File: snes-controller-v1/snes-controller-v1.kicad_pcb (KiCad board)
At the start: 2 copper layers, 66.1 x 20.1 mm, 19 parts, among them J1 USB_B_Micro, J2 NES, J3 Conn_01x06, J4 SNES_Controller_Socket, J5 SNES_Controller_Socket, U1 SN74LVC125ADR, U2 AP2112K-3.3, U7 ATSAMD21E18A-A

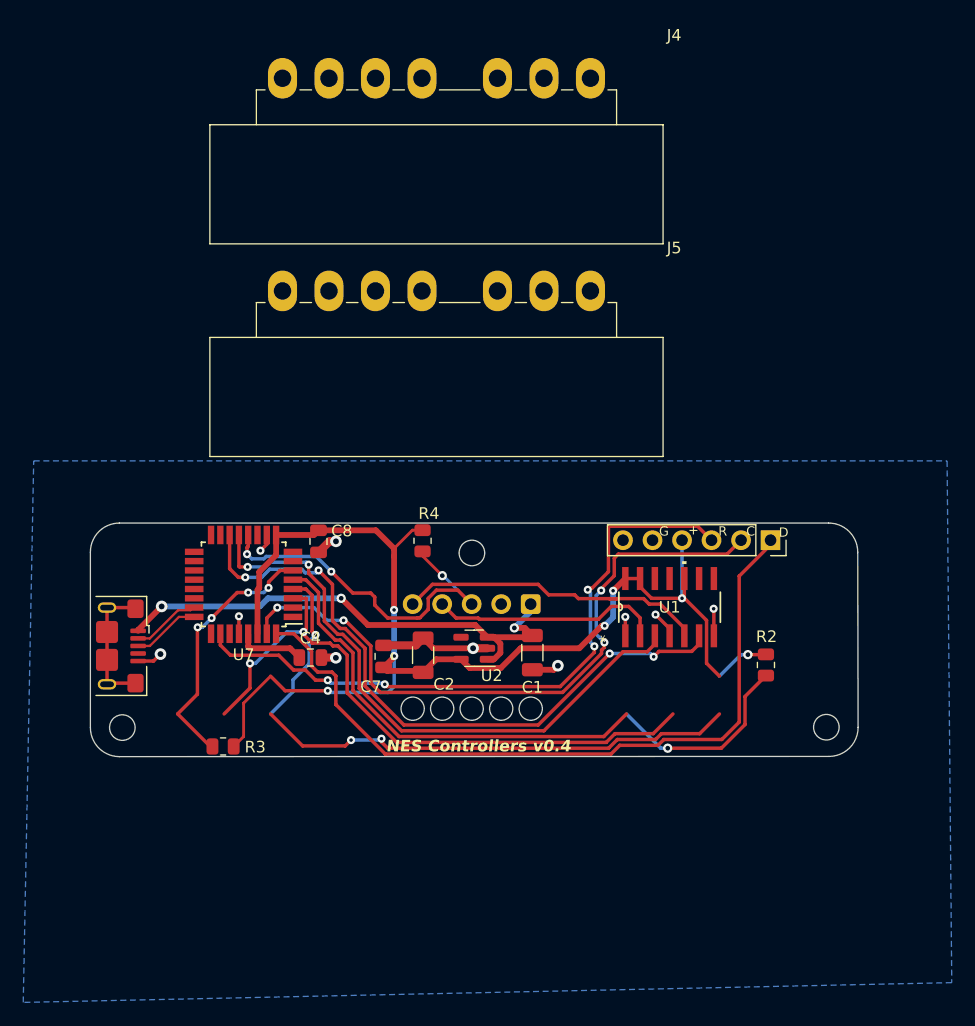
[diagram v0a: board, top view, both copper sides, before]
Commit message: ground plane
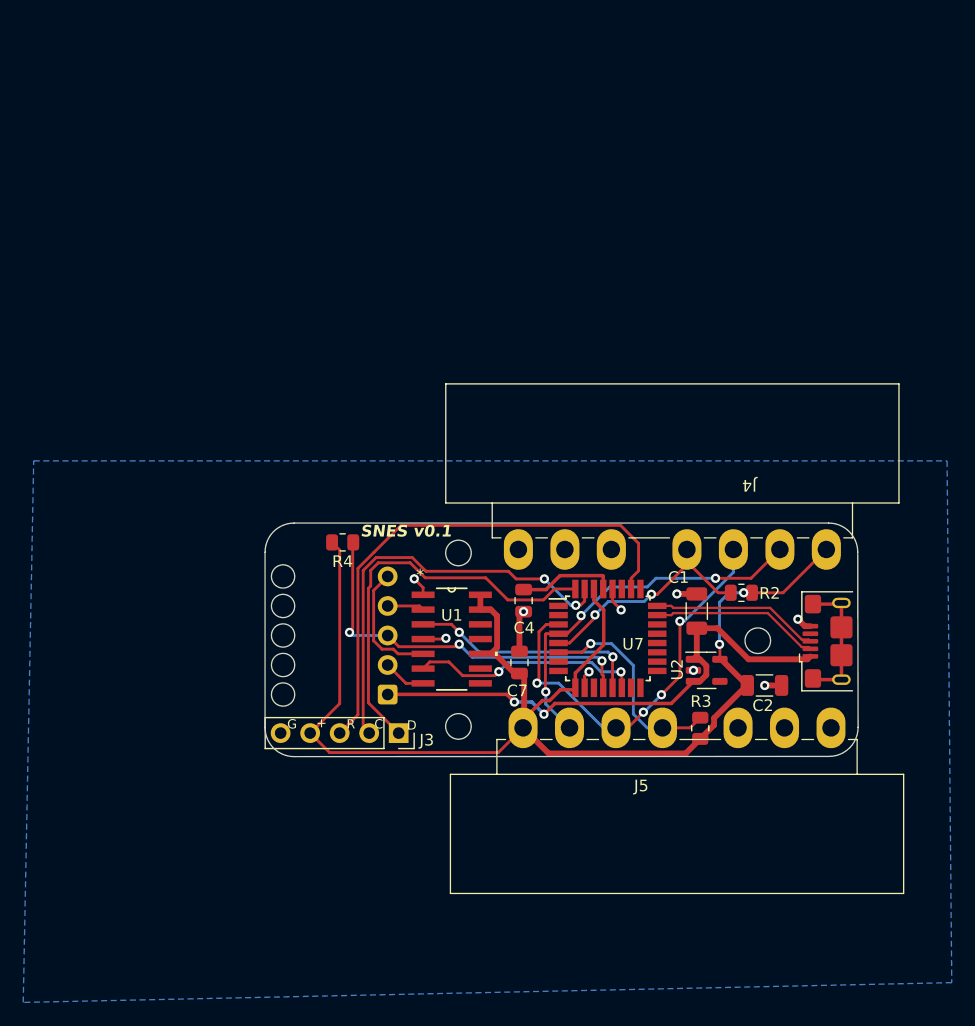
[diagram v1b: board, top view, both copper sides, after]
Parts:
- removed C8: 1uF, Capacitor_SMD:C_0805_2012Metric
- J3: value Conn_01x06 -> Conn_01x05; footprint Connector_PinSocket_2.54mm:PinSocket_1x06_P2.54mm_Vertical -> Connector_PinSocket_2.54mm:PinSocket_1x05_P2.54mm_Vertical
- moved J1 63.2 mm to (172.2, 74.4), turned to 90 degrees
- moved J4 61.9 mm to (170.9, 66.5), turned to 180 degrees
- moved J5 42.9 mm to (144.8, 81.9)
- moved R3 41.1 mm to (160.1, 81.9), turned to 90 degrees
- moved J3 36.0 mm to (134.1, 82.3)
- moved H1 32.6 mm to (139.2, 66.8)
- moved U7 31.7 mm to (152.1, 74.2), turned to 0 degrees
- moved C2 29.5 mm to (165.6, 78.2), turned to 0 degrees
- moved U2 20.1 mm to (160.6, 76.9), turned to 0 degrees
- moved C4 19.0 mm to (144.9, 70.9), turned to -90 degrees
- moved U1 18.9 mm to (138.7, 74.2), turned to 0 degrees
- moved H3 15.0 mm to (139.2, 81.8)
- moved C1 14.6 mm to (159.8, 71.8), turned to 90 degrees
- moved J2 14.6 mm to (133.2, 79.0), turned to 90 degrees
- moved C7 11.7 mm to (144.5, 76.2)
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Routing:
- net /NES_CLOCK_3V: track 57.2 -> 20.0 mm, vias 4 -> 2
- net /PAD_DATA_1: track 55.8 -> 21.2 mm, vias 1 -> 2
- net /NES_LATCH_3V: track 52.4 -> 20.2 mm
- net /SWDIO: track 64.2 -> 34.8 mm
- net /PAD_CLOCK: track 55.5 -> 32.3 mm
- net /SWCLK: track 57.6 -> 36.6 mm, vias 4 -> 2
- net /PAD_LATCH: track 53.9 -> 35.2 mm, vias 2 -> 4
- net /NES_LATCH_5V: track 20.7 -> 3.18 mm
- net /NES_CLOCK_5V: track 26.3 -> 11.1 mm
- net /RESET: track 57.2 -> 45.3 mm, vias 4 -> 0
- net /D-: track 5.82 -> 14.5 mm
- net /D+: track 5.76 -> 14.4 mm
- net GND: track 26.7 -> 19.1 mm, vias 10 -> 9
- net +3V3: track 107.3 -> 113.1 mm, vias 7 -> 2
- net /PAD_DATA_2: track 22.8 -> 18.3 mm, vias 4 -> 1
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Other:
- board size 66.1 x 20.1 mm -> 51 x 20.1 mm
- board text added: "SNES v0.1"
- board text removed: "NES Controllers v0.4"
